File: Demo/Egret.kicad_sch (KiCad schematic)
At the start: 24 parts, among them J1 Micro_SD_Card, Q1 S8050, Q2 S8050, U1 MPU6050, U2 LP2992IM5-3.3, U3 WS2812B-B, U4 CP2102N-A01-GQFN28, U5 ESP32-PICO-D4

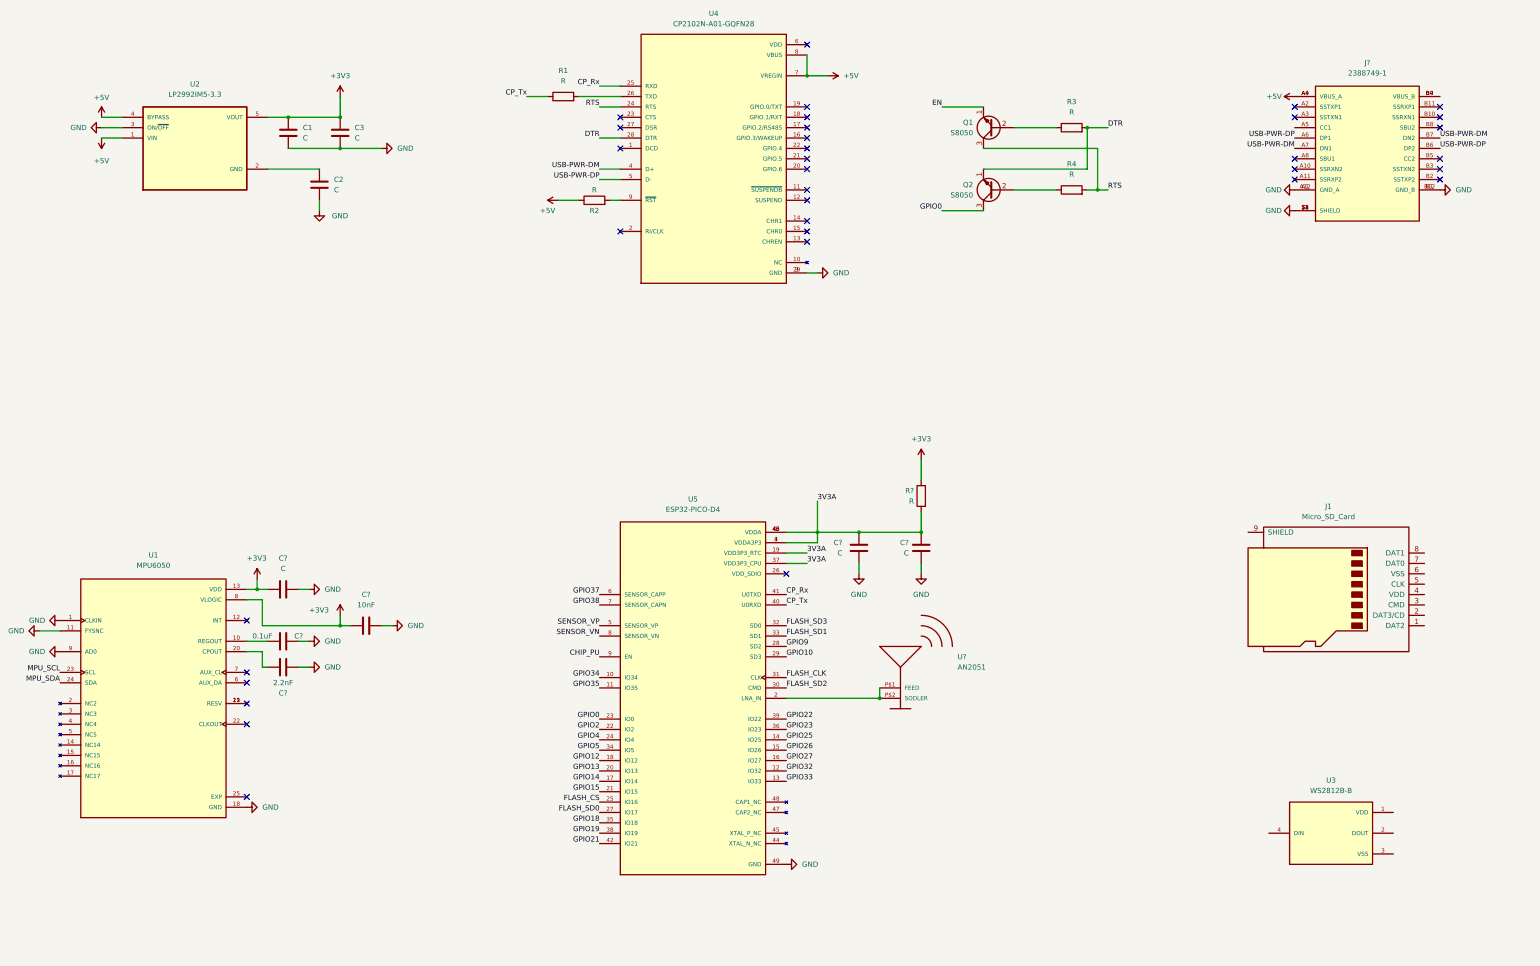
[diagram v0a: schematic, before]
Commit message: update
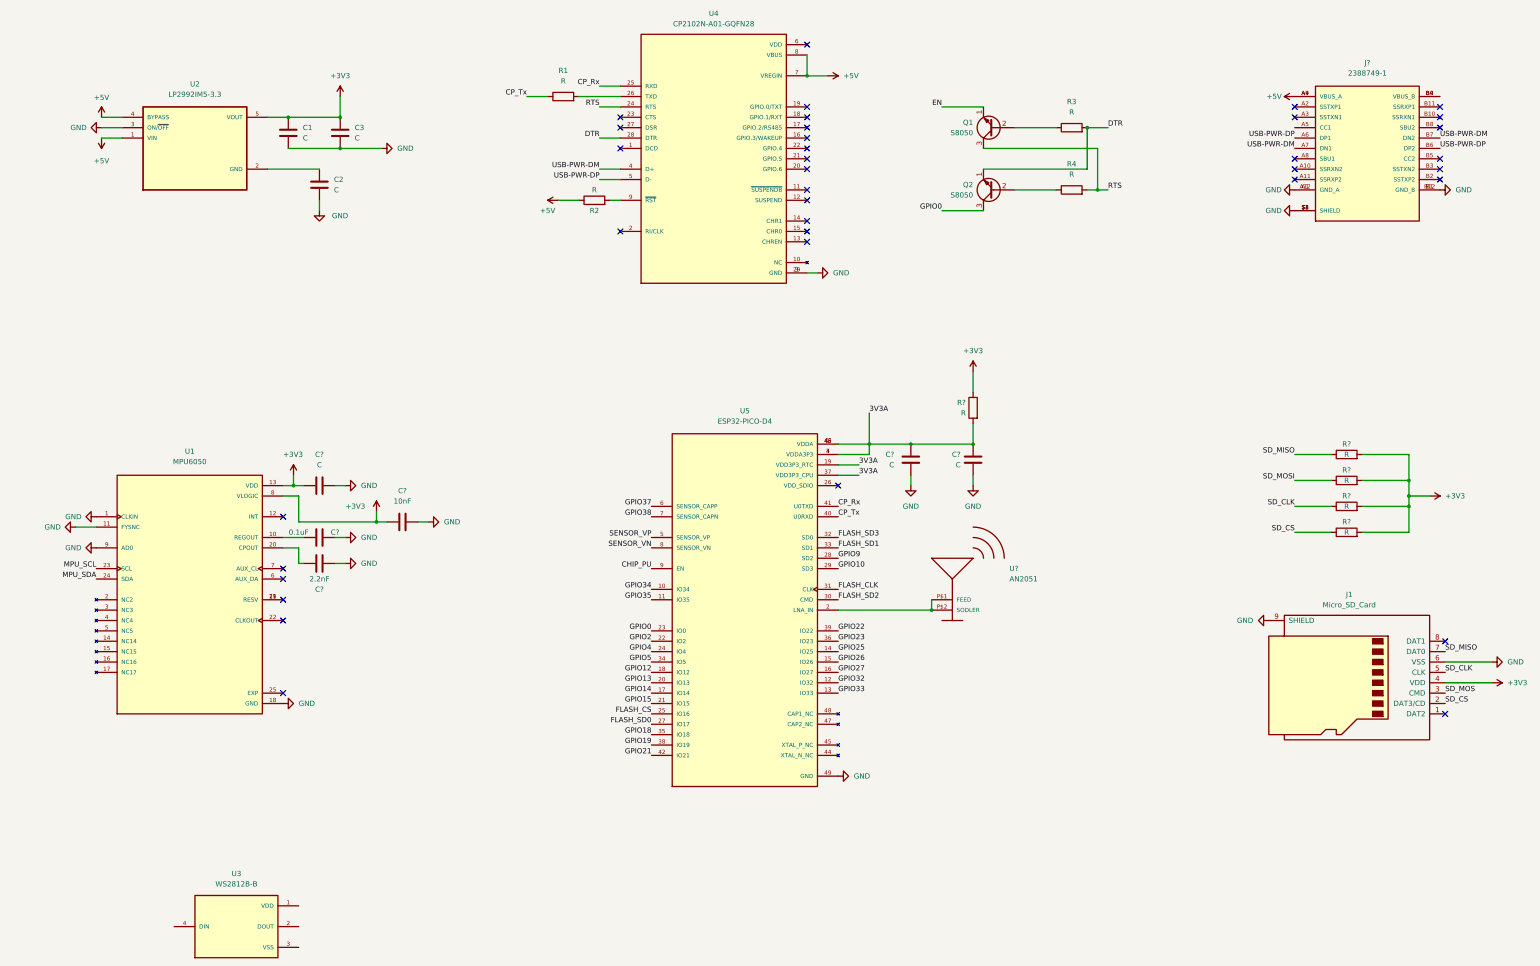
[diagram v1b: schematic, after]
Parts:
- added R? (x4): R, symbol Device:R
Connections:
- net +3V3: now also J1.4 (VDD), R?.2, R?.2, R?.2, R?.2
- net GND: now also J1.6 (VSS), J1.9 (SHIELD)
- net SD_CS: now reaches J1.2 (DAT3/CD)
- net SD_CS: now also R?.1
- net SD_MOS: now reaches J1.3 (CMD)
- net SD_CLK: now reaches J1.5 (CLK)
- net SD_CLK: now also R?.1
- net SD_MISO: now reaches J1.7 (DAT0)
- net SD_MISO: now also R?.1
- new net SD_MOSI: R?.1
- no-connect marks 35 -> 37
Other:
- moved on the sheet: C?, J1, R?, U1, U3, U5, U?
